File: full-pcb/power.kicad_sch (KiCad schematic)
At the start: 20 parts, among them J3 Barrel_Jack_Switch, U1 78L05G-AB3-R, U2 OPA1664D, U3 TPS5430DDA, U4 CJ431

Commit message: finished FFT sisplay test waiting for new PCB to arrive
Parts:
- L1: footprint Inductor_SMD:L_6.3x6.3_H3 -> Inductor_SMD:L_Changjiang_FNR8040S; MPN C20612510 -> C168130
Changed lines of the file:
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@@
 			)
 		)
-		(property "Footprint" "Inductor_SMD:L_6.3x6.3_H3"
+		(property "Footprint" "Inductor_SMD:L_Changjiang_FNR8040S"
 			(at 209.55 72.39 0)
 			(hide yes)
@@
 			)
 		)
-		(property "Datasheet" ""
+		(property "Datasheet" "C168130"
 			(at 209.55 72.39 0)
 			(hide yes)
@@
 			)
 		)
-		(property "MPN" "C20612510"
+		(property "MPN" "C168130"
 			(at 209.55 72.39 90)
 			(hide yes)

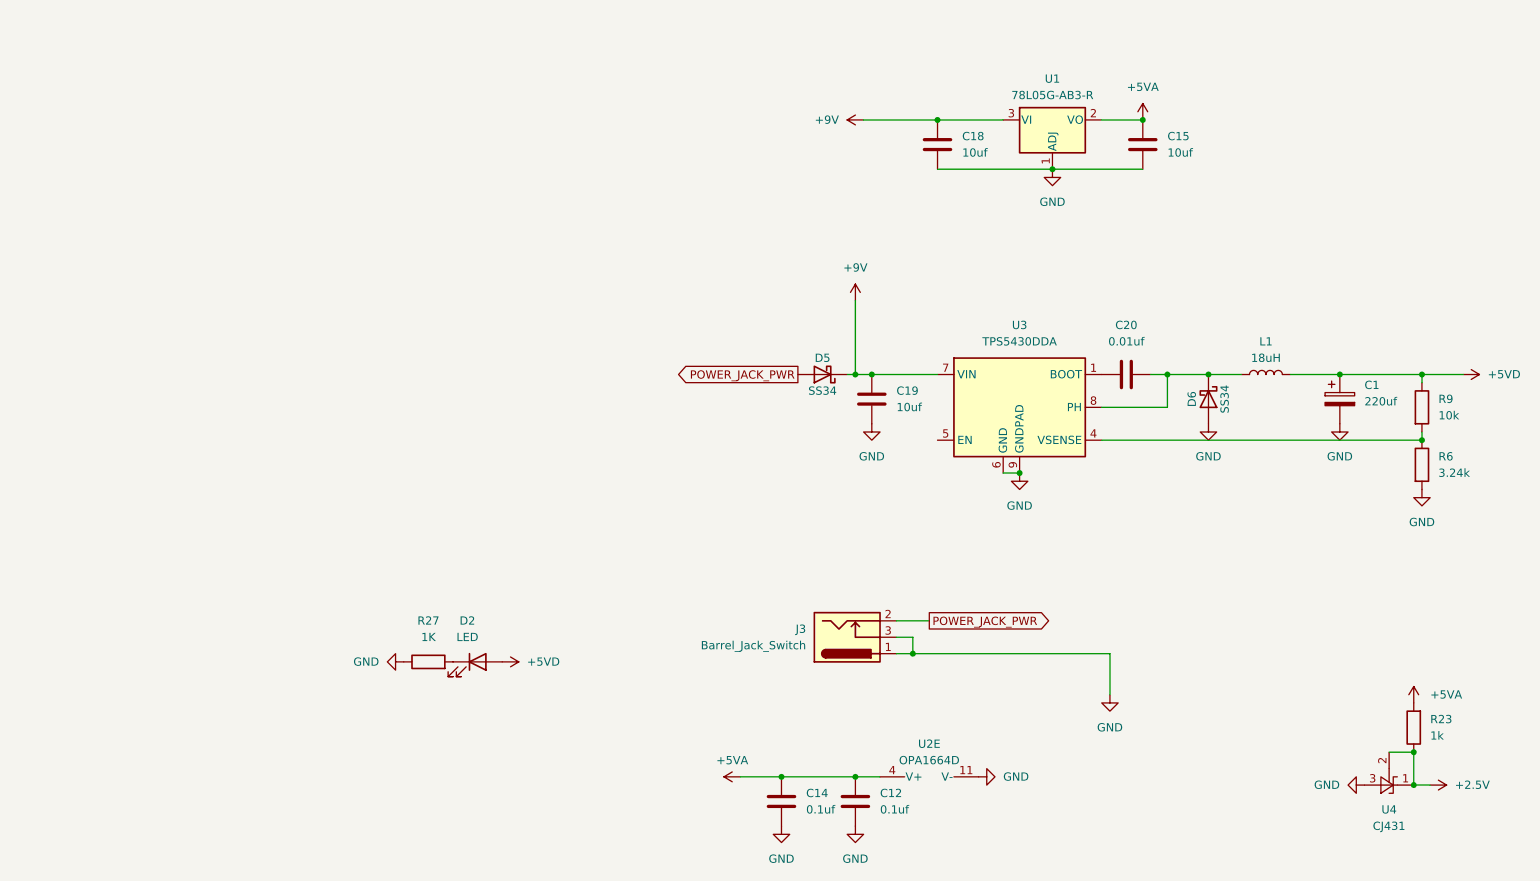
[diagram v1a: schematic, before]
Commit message: pedal works but is buggy
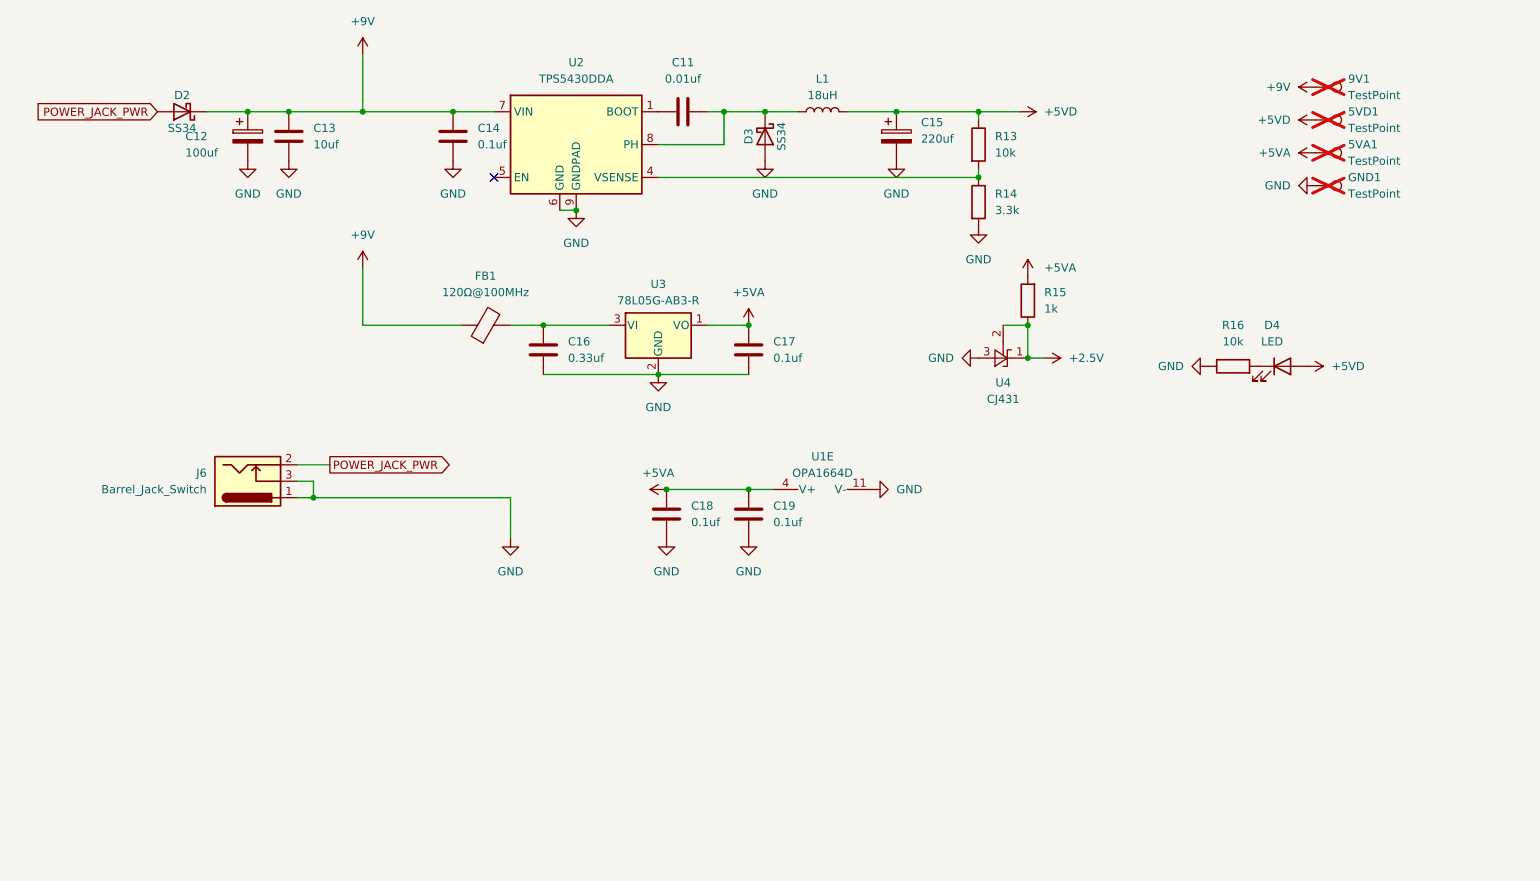
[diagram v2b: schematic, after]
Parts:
- removed C15: 10uf, Capacitor_SMD:C_0805_2012Metric, symbol Device:C
- removed R27: 1K, Resistor_SMD:R_0603_1608Metric, symbol Device:R
- added 5VA1, 5VD1, 9V1, GND1: TestPoint, Connector_PinHeader_2.54mm:PinHeader_1x01_P2.54mm_Vertical, symbol Connector:TestPoint
- added C12: 100uf, Capacitor_Tantalum_SMD:CP_EIA-3528-21_Kemet-B, symbol Device:C_Polarized
- added C16: 0.33uf, Capacitor_SMD:C_0805_2012Metric, symbol Device:C
- added C17: 0.1uf, Capacitor_SMD:C_0805_2012Metric, symbol Device:C
- added FB1: 120Ω@100MHz, Resistor_SMD:R_0603_1608Metric, symbol Device:FerriteBead
- added R16: 10k, Resistor_SMD:R_0603_1608Metric, symbol Device:R
- C18: value 10uf -> 0.1uf; MPN C440198 -> C49678
- R14: renamed from R6; value 3.24k -> 3.3k; MPN C166817 -> C22978
- U2: renamed from U3; MPN (none) -> C9864
- renumbered C20 to C11, C19 to C13, C1 to C15, C12 to C19, D5 to D2, D6 to D3, D2 to D4, J3 to J6, R9 to R13, R23 to R15, U2 to U1, U1 to U3
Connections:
- net +5VA: now also C18.1, U3.1 (VO), 5VA1.1, C17.2; no longer C14.1, U3.2 (VO)
- net +5VD: now also 5VD1.1
- net +9V: now also C14.2, 9V1.1, C12.1, FB1.1; no longer C18.2, U3.3 (VI)
- net GND: now also C14.1, C18.2, U3.2 (GND), C12.2, C16.1, C17.1, GND1.1, R16.1; no longer C14.2, C18.1, U3.1 (ADJ)
- net at D4.1 (K): now also R16.2
- new net: C16.2, FB1.2, U3.3 (VI)
- no-connect marks 0 -> 1
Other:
- moved on the sheet: C11, C13, C15, C19, D2, D3, D4, J6, L1, R13, R14, R15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
